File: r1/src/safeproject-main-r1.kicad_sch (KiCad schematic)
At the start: 14 parts, among them J1 2842142-4, J2 Conn_01x20

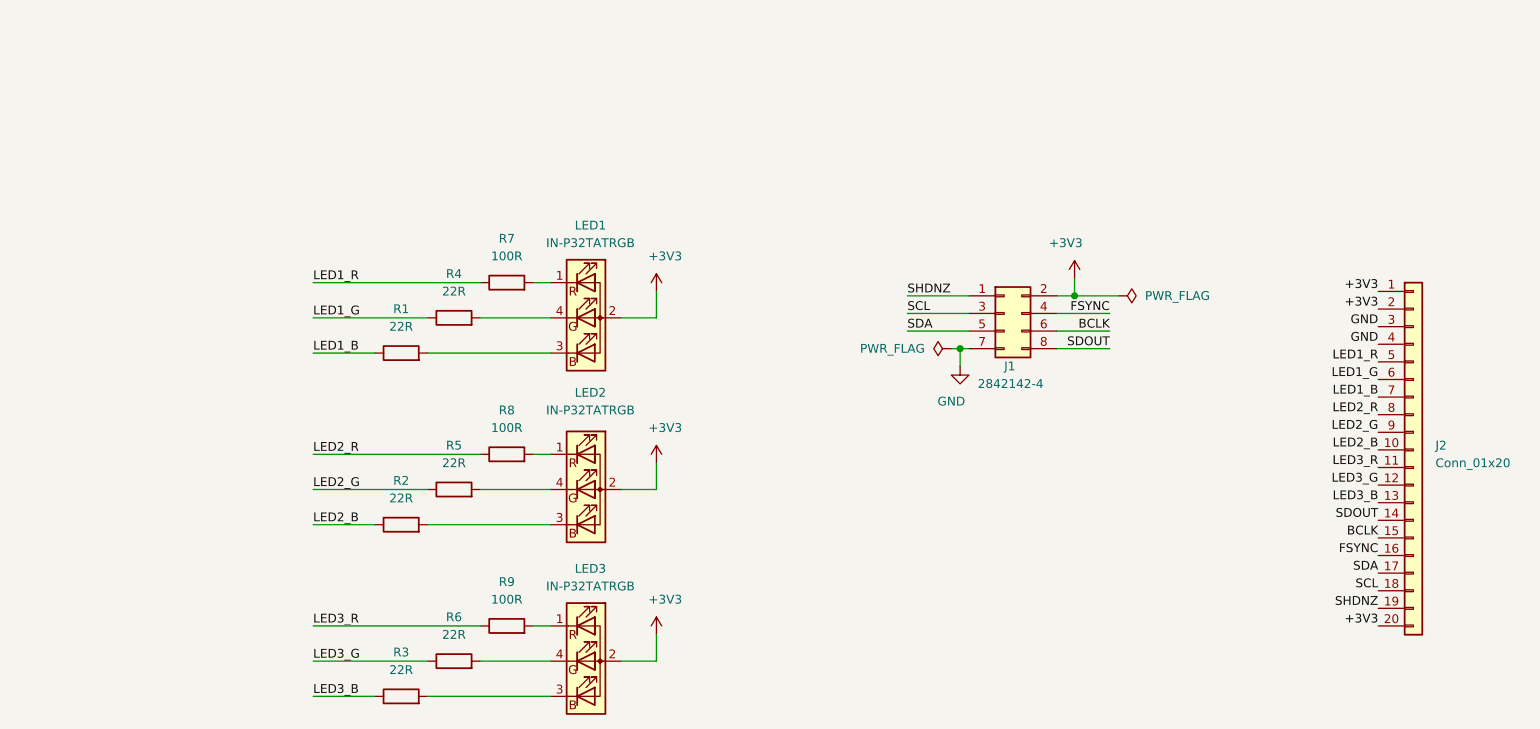
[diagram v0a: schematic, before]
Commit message: Board routed, DRC pass
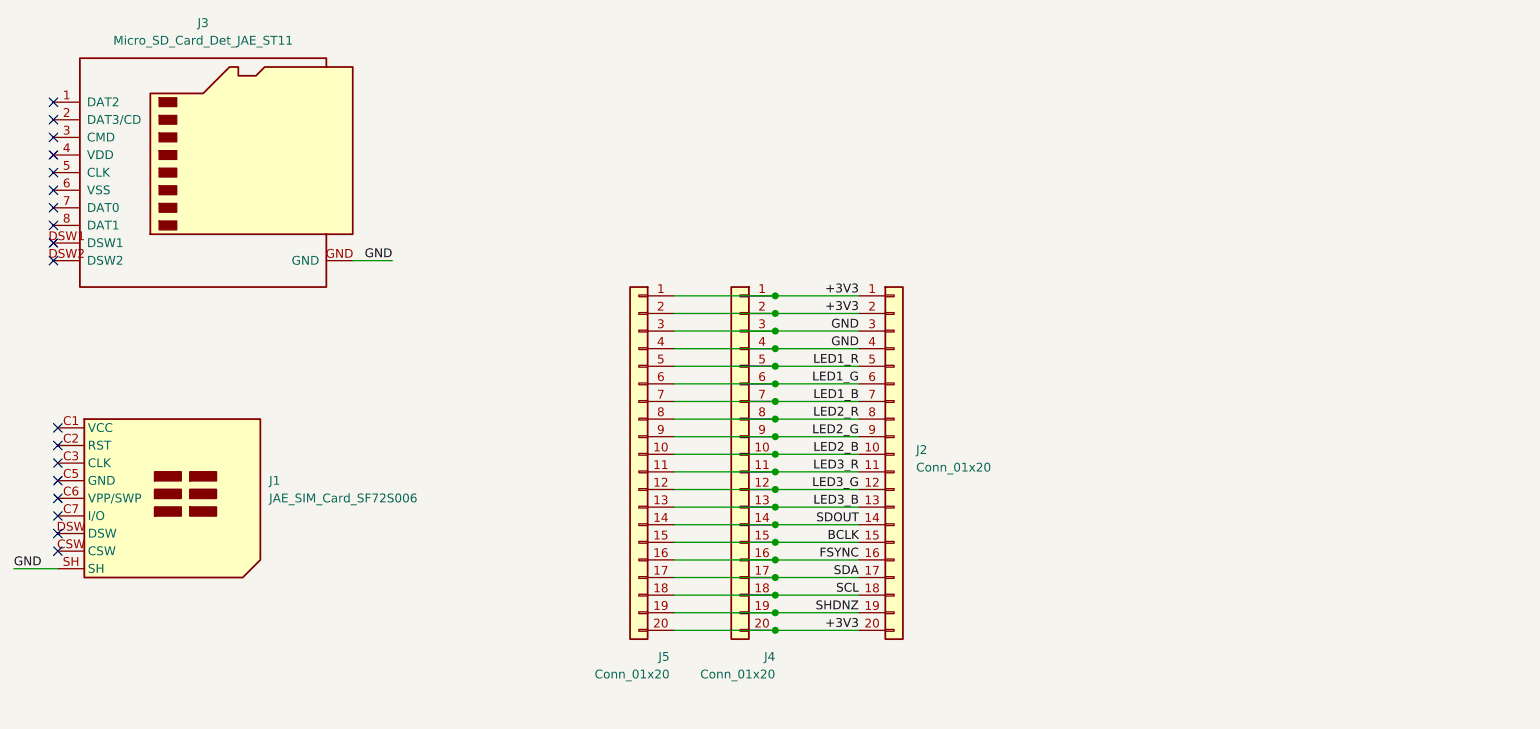
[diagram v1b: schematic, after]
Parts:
- removed J1: 2842142-4, jeffmakes-footprints:PinSocket_2x04_P2.00mm_Vertical_SMD_Bottom_or_Top_Entry_AMPMODU, symbol Connector_Generic:Conn_02x04_Odd_Even
- removed LED1, LED2, LED3: IN-P32TATRGB, LED_SMD:LED_Avago_PLCC4_3.2x2.8mm_CW, symbol Device:LED_RABG
- removed R1, R2, R3, R4, R5, R6: 22R, Resistor_SMD:R_0603_1608Metric, symbol Device:R
- removed R7, R8, R9: 100R, Resistor_SMD:R_0603_1608Metric, symbol Device:R
- added J1: JAE_SIM_Card_SF72S006, Connector_JAE:JAE_SIM_Card_SF72S006, symbol Connector:JAE_SIM_Card_SF72S006
- added J3: Micro_SD_Card_Det_JAE_ST11, jeffmakes-footprints:microSD_JAE_ST11S008V4H, symbol j_Connector:Micro_SD_Card_Det_JAE_ST11
- added J4: Conn_01x20, Connector_PinHeader_2.54mm:PinHeader_1x20_P2.54mm_Vertical_SMD_Pin1Right, symbol Connector_Generic:Conn_01x20
- added J5: Conn_01x20, Connector_PinHeader_2.54mm:PinHeader_1x20_P2.54mm_Vertical, symbol Connector_Generic:Conn_01x20
- J2: footprint Connector_FFC-FPC:Hirose_FH12-20S-0.5SH_1x20-1MP_P0.50mm_Horizontal -> jeffmakes-footprints:Hirose_FH12-20S-0.5SVA_1x20-1MP_P0.50mm_Vertical
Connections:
- net +3V3: now also J4.1 (Pin_1), J4.2 (Pin_2), J4.20 (Pin_20), J5.1 (Pin_1), J5.2 (Pin_2), J5.20 (Pin_20)
- net BCLK: now also J4.15 (Pin_15), J5.15 (Pin_15)
- net FSYNC: now also J4.16 (Pin_16), J5.16 (Pin_16)
- net GND: now also J1.SH, J3.GND, J4.3 (Pin_3), J4.4 (Pin_4), J5.3 (Pin_3), J5.4 (Pin_4)
- net LED1_B: now also J4.7 (Pin_7), J5.7 (Pin_7)
- net LED1_G: now also J4.6 (Pin_6), J5.6 (Pin_6)
- net LED1_R: now also J4.5 (Pin_5), J5.5 (Pin_5)
- net LED2_B: now also J4.10 (Pin_10), J5.10 (Pin_10)
- net LED2_G: now also J4.9 (Pin_9), J5.9 (Pin_9)
- net LED2_R: now also J4.8 (Pin_8), J5.8 (Pin_8)
- net LED3_B: now also J4.13 (Pin_13), J5.13 (Pin_13)
- net LED3_G: now also J4.12 (Pin_12), J5.12 (Pin_12)
- net LED3_R: now also J4.11 (Pin_11), J5.11 (Pin_11)
- net SCL: now also J4.18 (Pin_18), J5.18 (Pin_18)
- net SDA: now also J4.17 (Pin_17), J5.17 (Pin_17)
- net SDOUT: now also J4.14 (Pin_14), J5.14 (Pin_14)
- net SHDNZ: now also J4.19 (Pin_19), J5.19 (Pin_19)
- no-connect marks 0 -> 18
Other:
- moved on the sheet: J2
